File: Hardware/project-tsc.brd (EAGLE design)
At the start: 46 x 35 mm, 105 parts, among them IC1 BQ25180YBGR, IC2 DRV2605YZFR, IC3 BMA421, IC9 RT6160AWSC, J1 TC2030-IDC_TC2030-IDC, J2 503480-2400_503480-2400, J4 KH-TYPE-C-16P, Q1 20V/4.2A/52mΩ/1.4W, Q3 SI1308EDL-T1-GE3, U1 NRF52840_QF, U2 ESP32_C6_LIBRARY_MAX17048G+T10, X1 32MHz, X2 32.726kHz

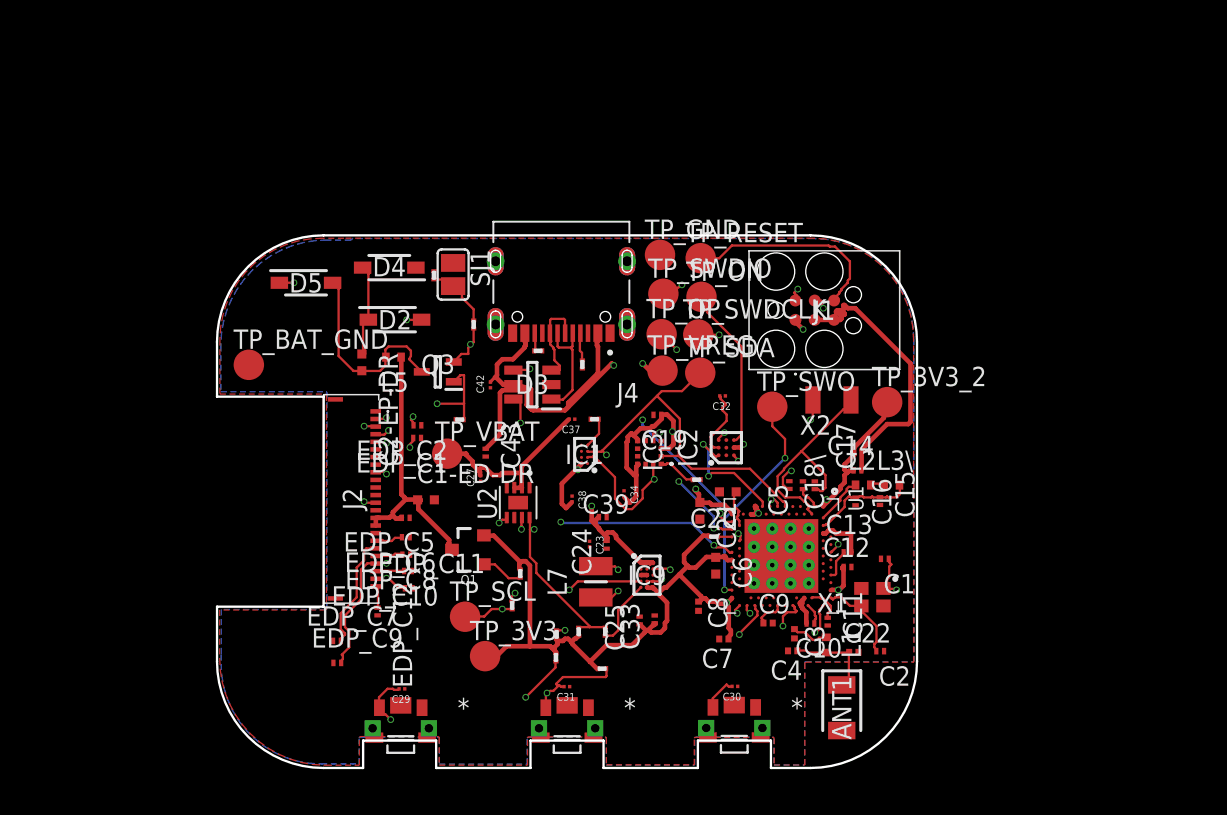
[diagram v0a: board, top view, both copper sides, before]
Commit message: Refactor code structure for improved readability and maintainability
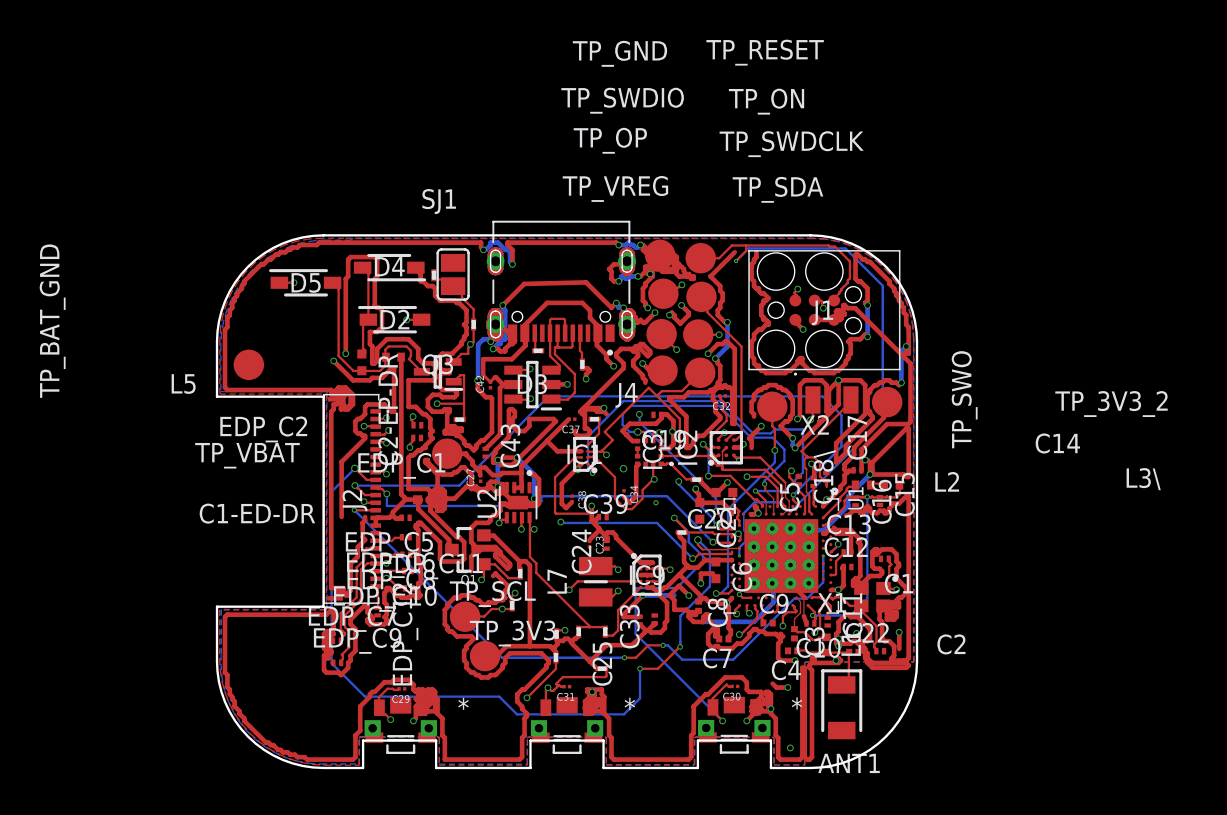
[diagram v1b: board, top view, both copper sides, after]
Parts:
- EDP_C1, EDP_C2: value 10uF -> 1uF
- R1, R2: value 10K -> 0
- moved R5 2.10 mm to (7.96, -1.74)
- moved C17 0.94 mm to (17.5, 1.91)
- moved C5 0.73 mm to (16.6, 1.57)
- moved C18\ 0.69 mm to (15.6, 1.67)
- moved C6 0.30 mm to (10.2, -4.23)
- moved C20 0.23 mm to (10.8, 0.88)
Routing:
- net GND: track 26.3 -> 805.8 mm, vias 0 -> 58
- net EPD_RST: track 0.00 -> 53.8 mm, vias 0 -> 4
- net EPD_CS: track 0.00 -> 45.1 mm, vias 0 -> 2
- net MOSI: track 0.00 -> 40.8 mm, vias 0 -> 4
- net RESET: track 13.9 -> 50.1 mm, vias 0 -> 2
- net P1.01: track 2.77 -> 32.6 mm, vias 0 -> 2
- net PMIC_INT: track 0.00 -> 27.7 mm, vias 0 -> 2
- net EPD_DC: track 0.00 -> 26.2 mm, vias 0 -> 2
- net P0.13: track 3.41 -> 28.0 mm, vias 0 -> 2
- net IMU_INT2: track 0.00 -> 20.5 mm, vias 0 -> 2
- net N$3: track 8.44 -> 20.1 mm, vias 0 -> 2
- net VREG: track 30.4 -> 38.6 mm
- net VBUS: track 51.7 -> 45.7 mm
- net SCL: track 49.9 -> 55.8 mm
- net 3V3: track 129.2 -> 125.6 mm
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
